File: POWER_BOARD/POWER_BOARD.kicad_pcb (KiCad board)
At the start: 2 copper layers, 41 parts, among them IC1 ILQ30, J2 ARM, J3 Pyro1, J4 Pyro2, J5 Servo2, J6 Servo1, J7 Batt, J9 505567-0671, Q1 IRL40B212, Q2 IRL40B212, U1 SF-1206HH10M-2, U2 SF-1206HH10M-2, U3 AS358AP

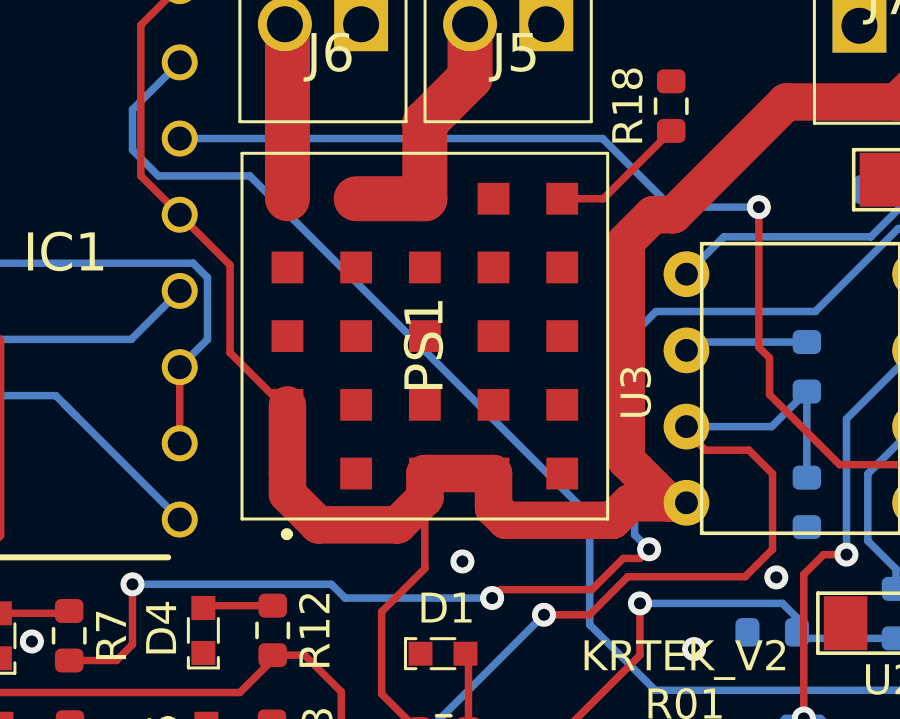
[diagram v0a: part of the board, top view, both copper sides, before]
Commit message: aaa
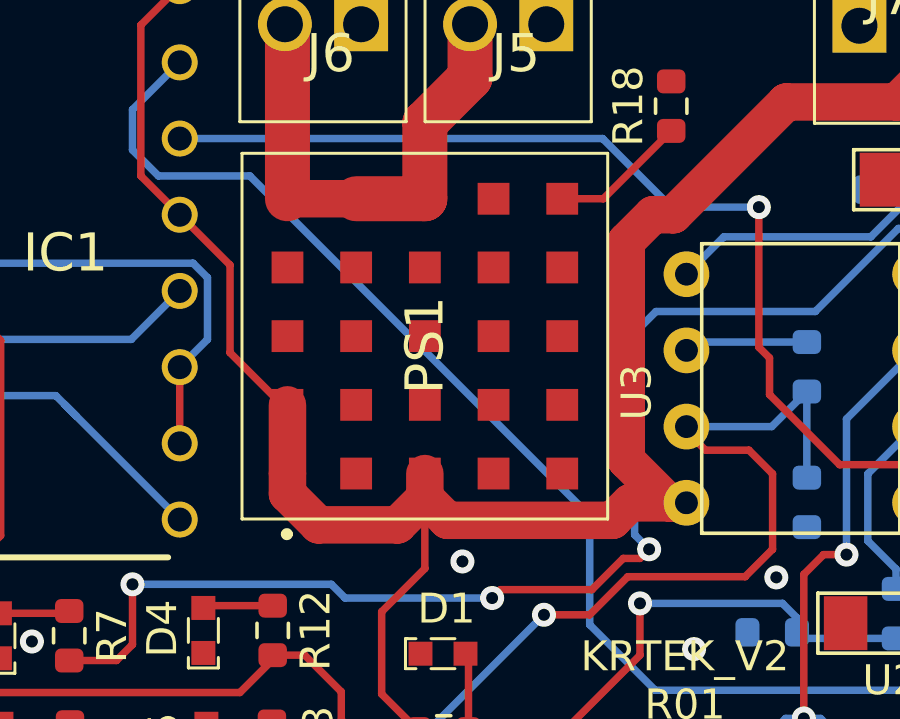
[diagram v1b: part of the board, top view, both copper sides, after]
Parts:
- J9: value 505567-0671 -> EXTIN
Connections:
- J6 pad 2: VINSERVO1 -> VINSERVO2
- PS1 pad A5: VINSERVO1 -> VINSERVO2
- PS1 pad D1: VCC -> Net-(PS1-PadD1)
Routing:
- net VINSERVO2: track 8.73 -> 16.9 mm
- net VINSERVO1: track 5.85 -> 0.00 mm
- net VCC: track 82.1 -> 81.1 mm
